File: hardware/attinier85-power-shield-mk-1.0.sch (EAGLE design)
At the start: 6 parts, among them IC1 MC34063DIP, U1 ATTINIER85_SHIELDV2

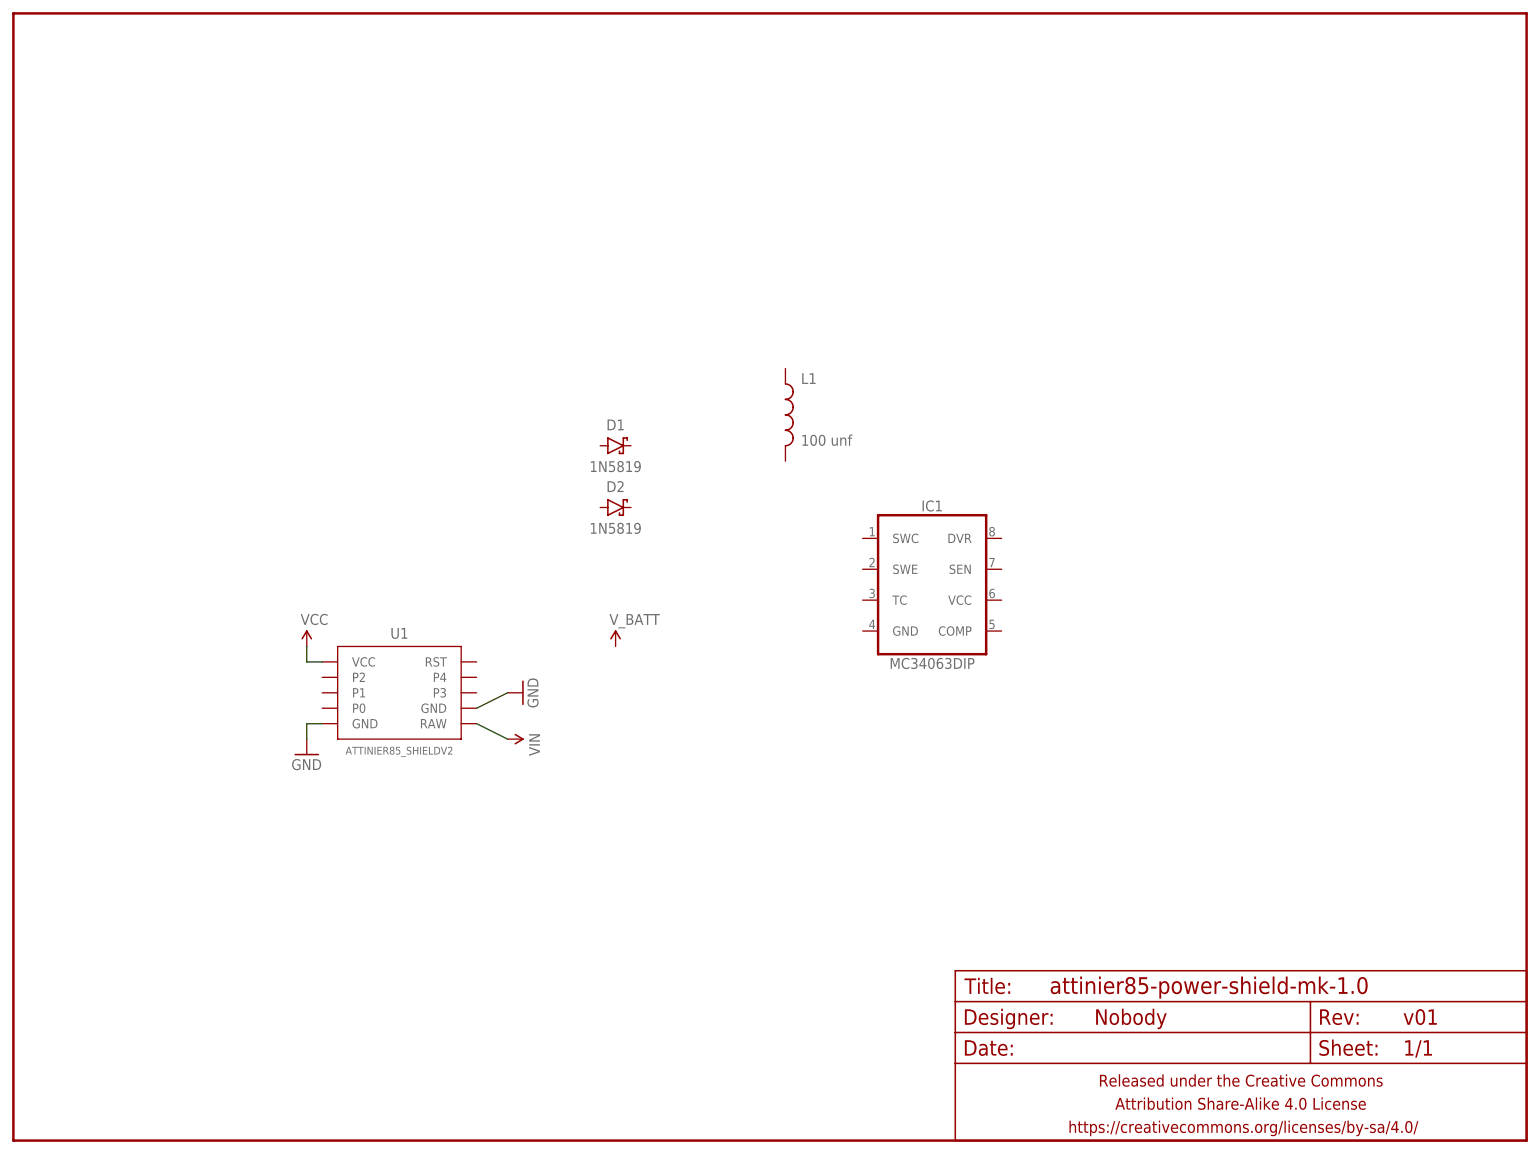
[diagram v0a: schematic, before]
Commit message: wooo
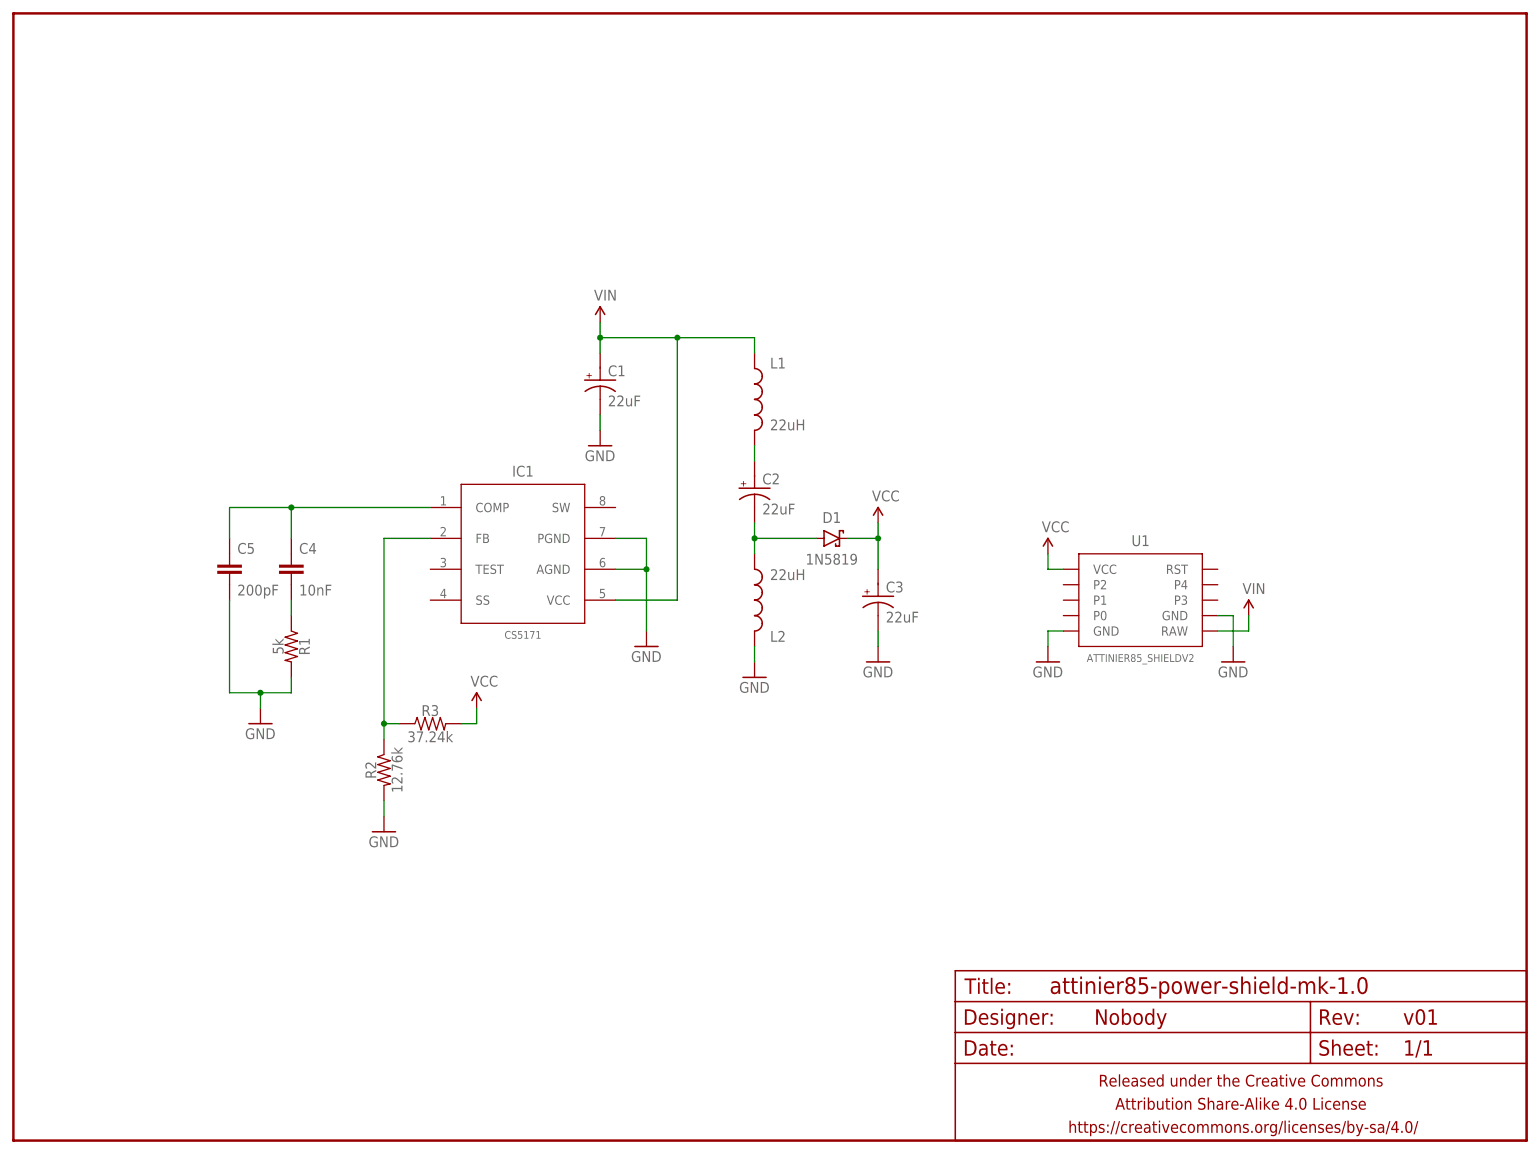
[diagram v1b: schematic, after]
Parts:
- removed D2: 1N5819, A_butts:DIODE-SCHOTTKYPTH-10.16MM
- added C1, C2, C3: 22uF, A_butts:CAPACITOR-POLARIZEDE2.5-6
- added C4: 10nF, A_butts:CAPACITOR-CERAMIC025-024X044
- added C5: 200pF, A_butts:CAPACITOR-CERAMIC025-024X044
- added L2: 22uH, A_butts:INDUCTORAXIAL-PTH-10.16MM
- added R1: 5k, A_butts:RESISTORPTH-AXIAL-6.35MM
- added R2: 12.76k, A_butts:RESISTORPTH-AXIAL-6.35MM
- added R3: 37.24k, A_butts:RESISTORPTH-AXIAL-6.35MM
- IC1: value MC34063DIP -> CS5171; device A_butts:MC34063DIP -> A_butts:CS5171/3SOIC-CS5171
- L1: value 100 unf -> 22uH
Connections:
- new net N$1: C4.2, R1.1
- new net N$3: C4.1, C5.1, IC1.COMP
- new net N$4: IC1.FB, R2.1, R3.1
- new net N$6: C2.+, L1.2
- new net N$7: C2.-, D1.A, L2.2
- net GND: now also C1.-, C3.-, C5.2, IC1.AGND, IC1.PGND, L2.1, R1.2, R2.2
- net VCC: now also C3.+, D1.C, R3.2
- net VIN: now also C1.+, IC1.VCC, L1.1
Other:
- moved on the sheet: D1, IC1, L1, U1
